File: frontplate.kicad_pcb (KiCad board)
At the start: 2 copper layers, 200 x 105 mm, 5 parts

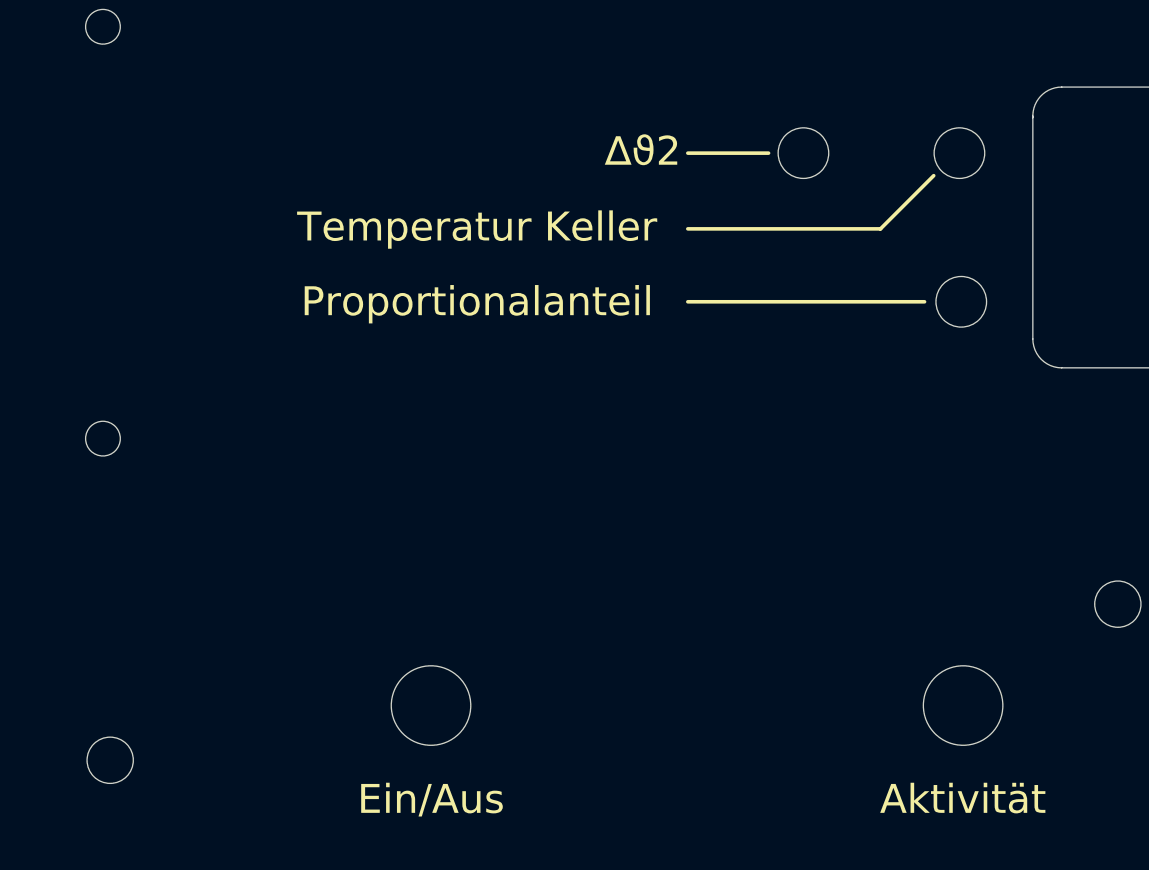
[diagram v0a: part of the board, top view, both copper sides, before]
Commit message: Production state Rev.B
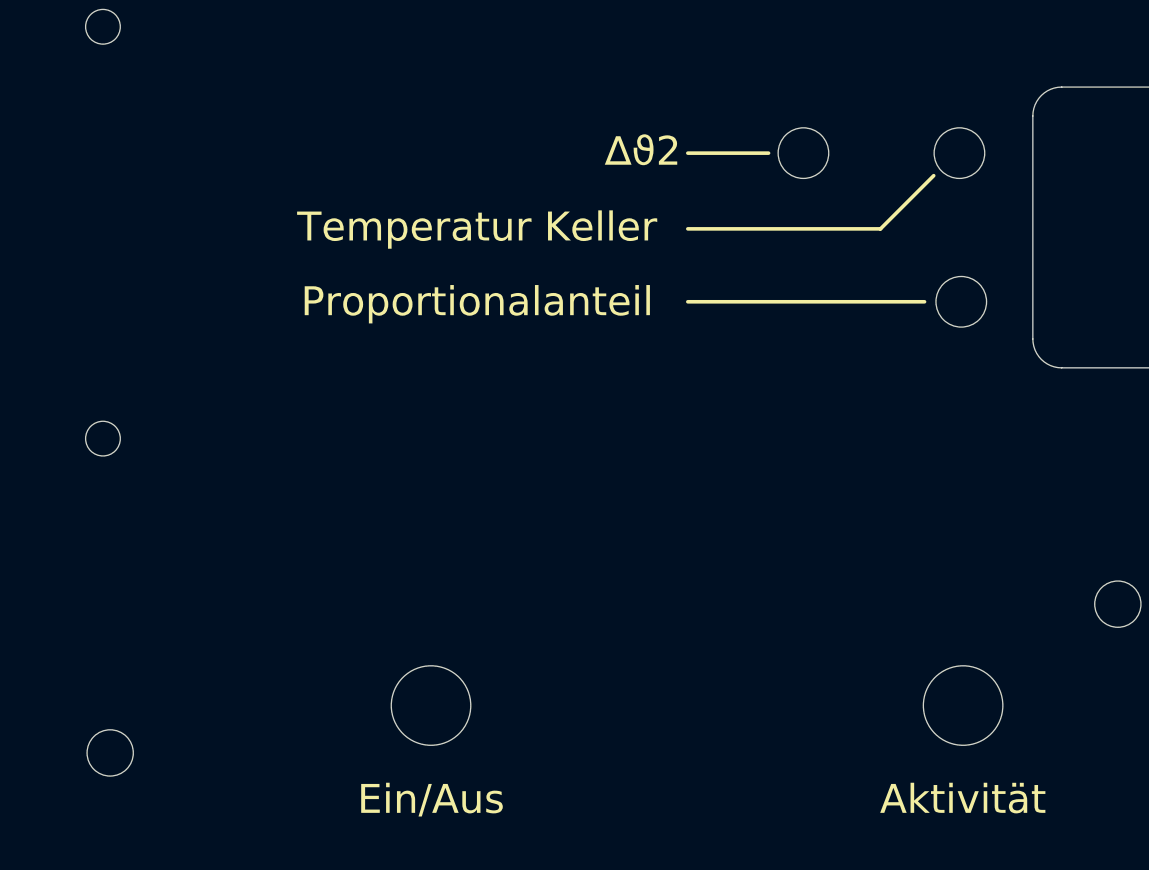
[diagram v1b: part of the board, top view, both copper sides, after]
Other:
- outline, holes or cut-outs redrawn
- board text added: "Reichelt: "SK M3" as nuts (x6)"
- board text added: "Reichelt: "SZK M3X6-200" as screws (x6)"
- board text added: "Reichelt: "VT DA 12MM" as distance bolts (x6)"
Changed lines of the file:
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@@
   (general
     (thickness 1.6)
-    (drawings 65)
+    (drawings 68)
     (tracks 0)
     (zones 0)
@@
   (page A4)
   (layers
-    (0 F.Cu signal)
+    (0 F.Cu signal hide)
     (31 B.Cu signal)
     (32 B.Adhes user hide)
@@
       (drillshape 0)
       (scaleselection 1)
-      (outputdirectory "C:/Users/stoff/source/repos/solaranlage/Production Files/GER/"))
+      (outputdirectory "C:/Users/mstof/source/repos/solaranlage/Production Files/Rev_B/GER/frontpalte"))
   )
   (net 0 "")
@@
     )
   )
+  (gr_text "Reichelt: \"SK M3\" as nuts (x6)" (at 75.820286 182.0545) (layer Eco2.User)
+    (effects (font (size 3 3) (thickness 0.15)))
+  )
+  (gr_text "Reichelt: \"VT DA 12MM\" as distance bolts (x6)" (at 93.748857 177.165) (layer Eco2.User)
+    (effects (font (size 3 3) (thickness 0.15)))
+  )
+  (gr_text "Reichelt: \"SZK M3X6-200\" as screws (x6)" (at 88.963143 171.8945) (layer Eco2.User)
+    (effects (font (size 3 3) (thickness 0.15)))
+  )
   (gr_arc (start 156.75 105.061) (end 156.75 107.061) (angle -90) (layer Edge.Cuts) (width 0.05))
   (gr_arc (start 121.126 105.061) (end 119.126 105.061) (angle -90) (layer Edge.Cuts) (width 0.05))
   (gr_arc (start 156.75 89.63) (end 158.75 89.63) (angle -90) (layer Edge.Cuts) (width 0.05))
-  (gr_arc (start 121.126 89.63) (end 121.126 87.63) (angle -93.6) (layer Edge.Cuts) (width 0.05))
+  (gr_arc (start 121.126 89.63) (end 121.126 87.63) (angle -90) (layer Edge.Cuts) (width 0.05))
   (gr_arc (start 156.75 78.391) (end 156.75 80.391) (angle -90) (layer Edge.Cuts) (width 0.05))
   (gr_arc (start 121.126 78.391) (end 119.126 78.391) (angle -90) (layer Edge.Cuts) (width 0.05))
@@
   (gr_circle (center 222.588 61.708) (end 224.188 61.708) (layer Edge.Cuts) (width 0.05))
   (gr_circle (center 43.433 145.708) (end 45.033 145.708) (layer Edge.Cuts) (width 0.05))
-  (gr_circle (center 55.278 134.216) (end 56.878 134.216) (layer Edge.Cuts) (width 0.05))
+  (gr_circle (center 55.278 133.708) (end 56.878 133.708) (layer Edge.Cuts) (width 0.05))
   (gr_circle (center 43.433 49.708) (end 45.033 49.708) (layer Edge.Cuts) (width 0.05))
   (gr_circle (center 55.278 61.708) (end 56.878 61.708) (layer Edge.Cuts) (width 0.05))
@@
     (connect_pads (clearance 0.508))
     (min_thickness 0.254)
-    (fill yes (arc_segments 32) (thermal_gap 0.508) (thermal_bridge_width 0.508))
+    (fill (arc_segments 32) (thermal_gap 0.508) (thermal_bridge_width 0.508))
     (polygon
       (pts
@@
     (connect_pads (clearance 0.508))
     (min_thickness 0.254)
-    (fill yes (arc_segments 32) (thermal_gap 0.508) (thermal_bridge_width 0.508))
+    (fill (arc_segments 32) (thermal_gap 0.508) (thermal_bridge_width 0.508))
     (polygon
       (pts
